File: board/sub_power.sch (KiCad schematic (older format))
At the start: 1 part, among them U201 XC3S200-TQ144

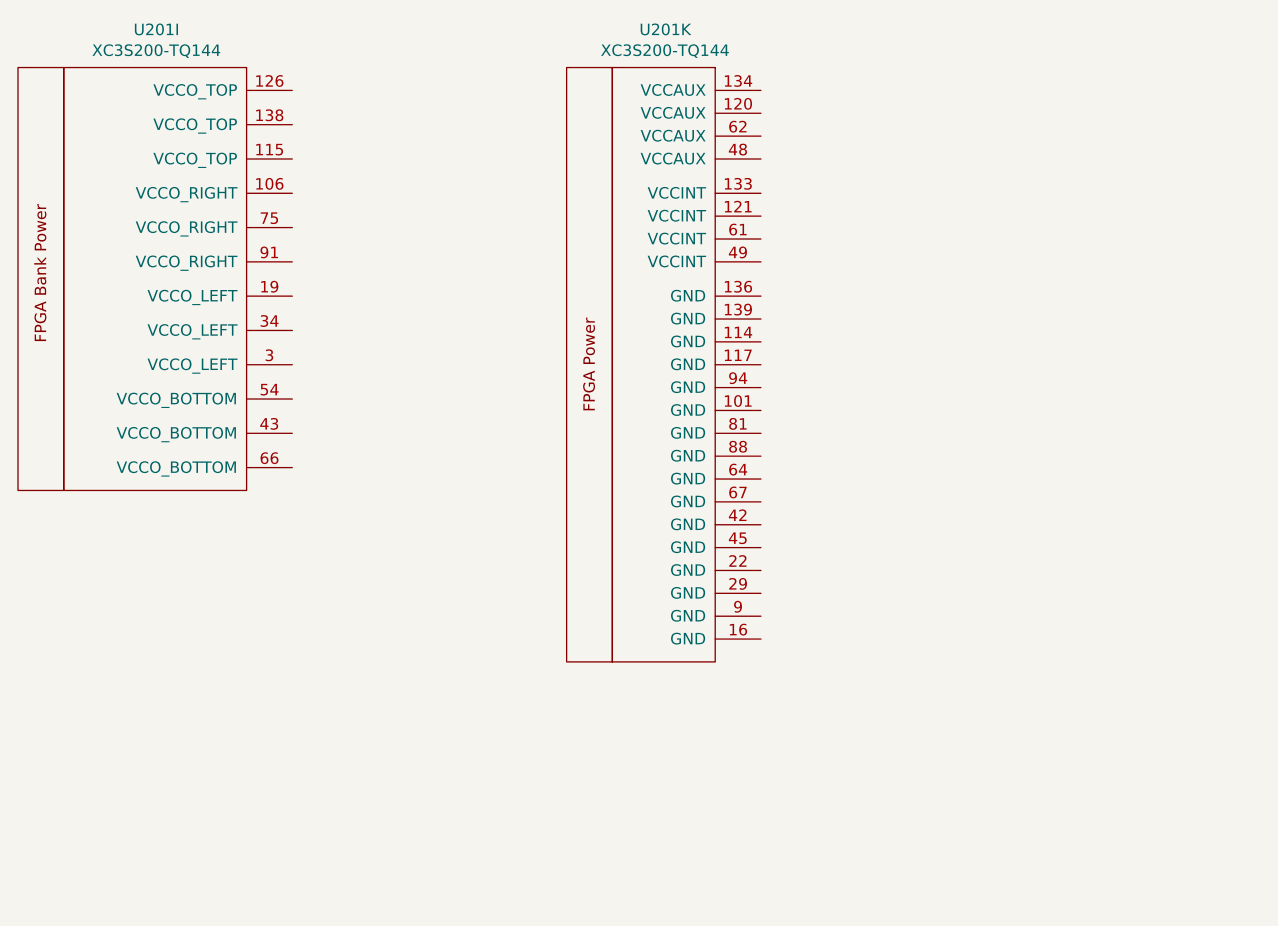
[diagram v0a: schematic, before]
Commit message: More schematic progress
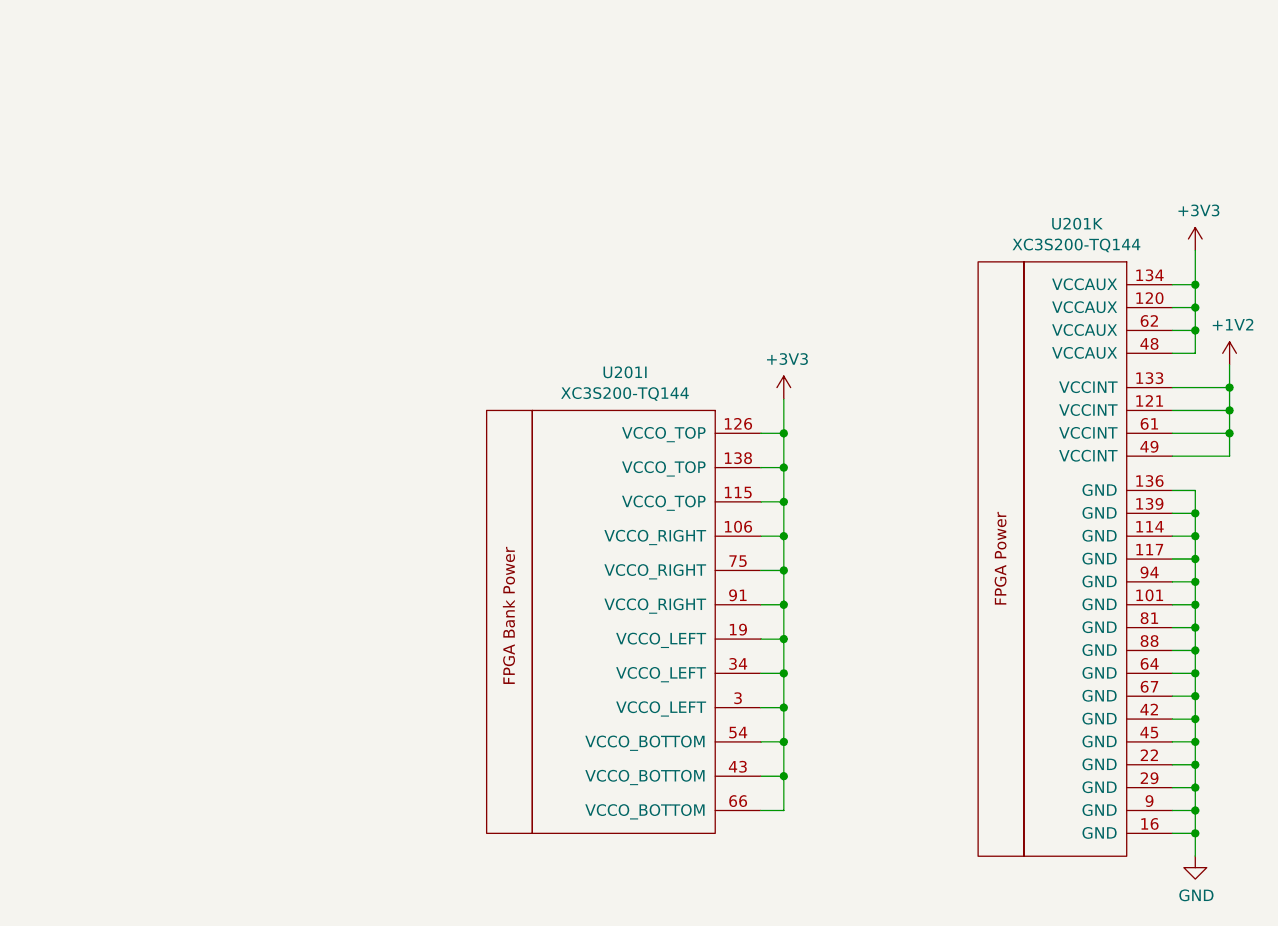
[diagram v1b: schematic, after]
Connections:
- net +3V3: now reaches U201.106 (VCCO_RIGHT)
- net +3V3: now also U201.115 (VCCO_TOP), U201.120 (VCCAUX), U201.126 (VCCO_TOP), U201.134 (VCCAUX), U201.138 (VCCO_TOP), U201.19 (VCCO_LEFT), U201.3 (VCCO_LEFT), U201.34 (VCCO_LEFT), U201.43 (VCCO_BOTTOM), U201.48 (VCCAUX), U201.54 (VCCO_BOTTOM), U201.62 (VCCAUX), U201.66 (VCCO_BOTTOM), U201.75 (VCCO_RIGHT), U201.91 (VCCO_RIGHT)
- net GND: now reaches U201.101 (GND)
- net GND: now also U201.114 (GND), U201.117 (GND), U201.136 (GND), U201.139 (GND), U201.16 (GND), U201.22 (GND), U201.29 (GND), U201.42 (GND), U201.45 (GND), U201.64 (GND), U201.67 (GND), U201.81 (GND), U201.88 (GND), U201.9 (GND), U201.94 (GND)
- net +1V2: now reaches U201.121 (VCCINT)
- net +1V2: now also U201.133 (VCCINT), U201.49 (VCCINT), U201.61 (VCCINT)
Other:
- moved on the sheet: U201I, U201K
